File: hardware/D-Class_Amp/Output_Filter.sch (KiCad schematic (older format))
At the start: 4 parts

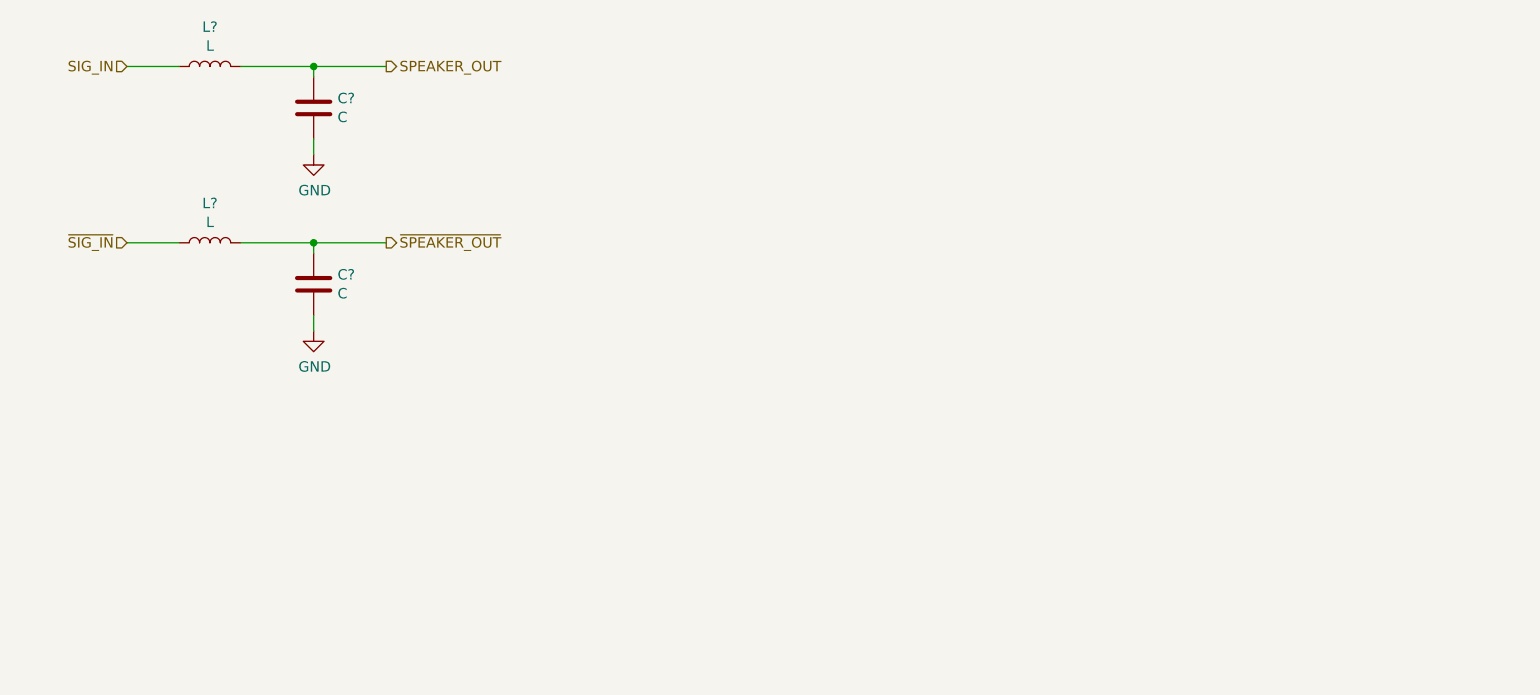
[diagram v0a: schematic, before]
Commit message: single side
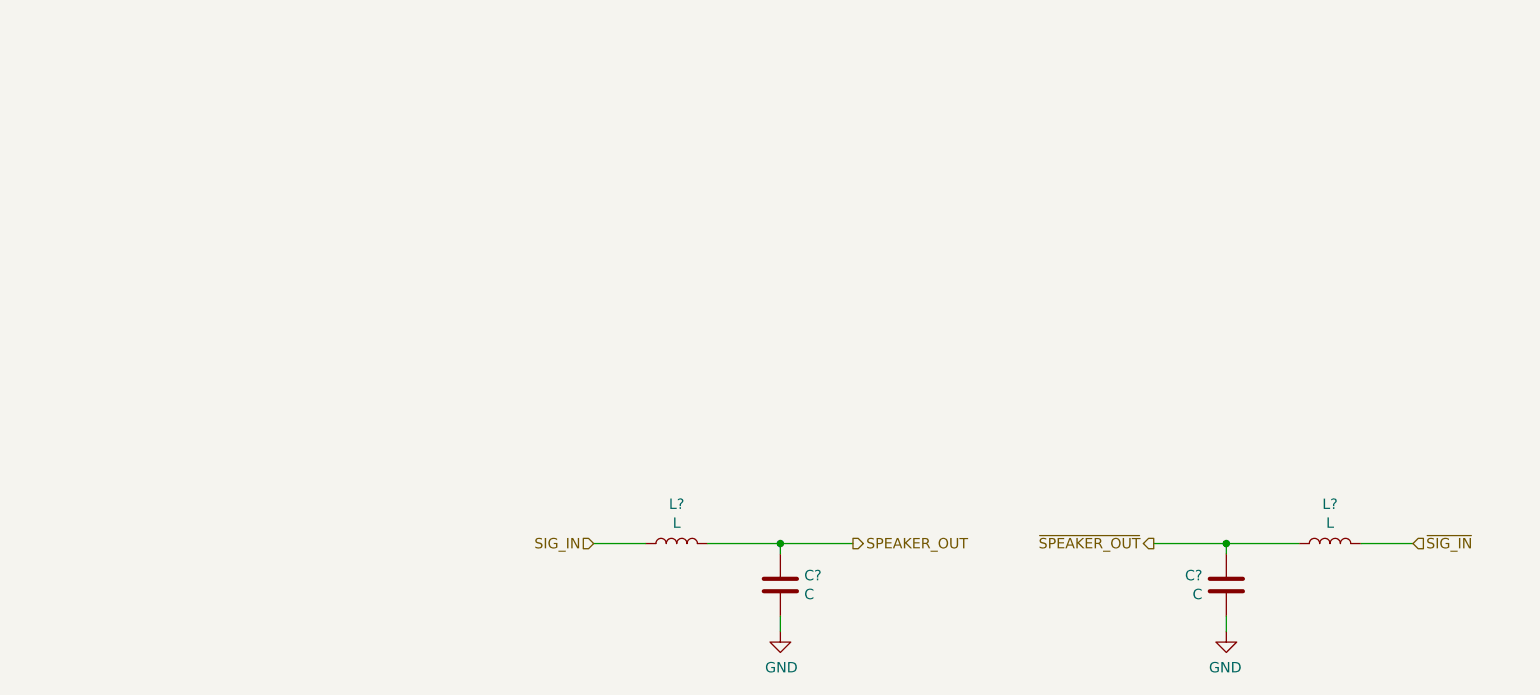
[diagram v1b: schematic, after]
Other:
- moved on the sheet: C?, L?
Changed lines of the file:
@@
 Comment4 ""
 $EndDescr
-Text HLabel 1450 1200 0    50   Input ~ 0
+Text HLabel 3700 3500 0    50   Input ~ 0
 SIG_IN
-Text HLabel 1450 2050 0    50   Input ~ 0
+Text HLabel 7650 3500 2    50   Input ~ 0
 ~SIG_IN
 $Comp
 L Device:L L?
 U 1 1 61193FAD
-P 1850 1200
-F 0 "L?" V 2040 1200 50  0000 C CNN
-F 1 "L" V 1949 1200 50  0000 C CNN
-F 2 "" H 1850 1200 50  0001 C CNN
-F 3 "~" H 1850 1200 50  0001 C CNN
-	1    1850 1200
+P 4100 3500
+F 0 "L?" V 4290 3500 50  0000 C CNN
+F 1 "L" V 4199 3500 50  0000 C CNN
+F 2 "" H 4100 3500 50  0001 C CNN
+F 3 "~" H 4100 3500 50  0001 C CNN
+	1    4100 3500
 	0    -1   -1   0
 $EndComp
@@
 L Device:L L?
 U 1 1 61195264
-P 1850 2050
-F 0 "L?" V 2040 2050 50  0000 C CNN
-F 1 "L" V 1949 2050 50  0000 C CNN
-F 2 "" H 1850 2050 50  0001 C CNN
-F 3 "~" H 1850 2050 50  0001 C CNN
-	1    1850 2050
-	0    -1   -1   0
+P 7250 3500
+F 0 "L?" V 7440 3500 50  0000 C CNN
+F 1 "L" V 7349 3500 50  0000 C CNN
+F 2 "" H 7250 3500 50  0001 C CNN
+F 3 "~" H 7250 3500 50  0001 C CNN
+	1    7250 3500
+	0    1    -1   0
 $EndComp
 $Comp
 L Device:C C?
 U 1 1 611955B4
-P 2350 1400
-F 0 "C?" H 2465 1446 50  0000 L CNN
-F 1 "C" H 2465 1355 50  0000 L CNN
-F 2 "" H 2388 1250 50  0001 C CNN
-F 3 "~" H 2350 1400 50  0001 C CNN
-	1    2350 1400
+P 4600 3700
+F 0 "C?" H 4715 3746 50  0000 L CNN
+F 1 "C" H 4715 3655 50  0000 L CNN
+F 2 "" H 4638 3550 50  0001 C CNN
+F 3 "~" H 4600 3700 50  0001 C CNN
+	1    4600 3700
 	1    0    0    -1
 $EndComp
@@
 L Device:C C?
 U 1 1 61195DF7
-P 2350 2250
-F 0 "C?" H 2465 2296 50  0000 L CNN
-F 1 "C" H 2465 2205 50  0000 L CNN
-F 2 "" H 2388 2100 50  0001 C CNN
-F 3 "~" H 2350 2250 50  0001 C CNN
-	1    2350 2250
-	1    0    0    -1
+P 6750 3700
+F 0 "C?" H 6865 3746 50  0000 L CNN
+F 1 "C" H 6865 3655 50  0000 L CNN
+F 2 "" H 6788 3550 50  0001 C CNN
+F 3 "~" H 6750 3700 50  0001 C CNN
+	1    6750 3700
+	-1   0    0    -1
 $EndComp
 Wire Wire Line
-	1450 1200 1700 1200
+	3700 3500 3950 3500
 Wire Wire Line
-	2000 1200 2350 1200
+	4250 3500 4600 3500
 Wire Wire Line
-	2350 1200 2350 1250
+	4600 3500 4600 3550
 Wire Wire Line
-	2350 1200 2700 1200
-Connection ~ 2350 1200
+	4600 3500 4950 3500
+Connection ~ 4600 3500
 Wire Wire Line
-	1450 2050 1700 2050
+	7650 3500 7400 3500
 Wire Wire Line
-	2000 2050 2350 2050
+	7100 3500 6750 3500
 Wire Wire Line
-	2350 2050 2350 2100
+	6750 3500 6750 3550
 Wire Wire Line
-	2350 2050 2700 2050
-Connection ~ 2350 2050
+	6750 3500 6400 3500
+Connection ~ 6750 3500
 $Comp
 L power:GND #PWR?
 U 1 1 611D879A
-P 2350 1625
-F 0 "#PWR?" H 2350 1375 50  0001 C CNN
-F 1 "GND" H 2355 1452 50  0000 C CNN
-F 2 "" H 2350 1625 50  0001 C CNN
-F 3 "" H 2350 1625 50  0001 C CNN
-	1    2350 1625
+P 4600 3925
+F 0 "#PWR?" H 4600 3675 50  0001 C CNN
+F 1 "GND" H 4605 3752 50  0000 C CNN
+F 2 "" H 4600 3925 50  0001 C CNN
+F 3 "" H 4600 3925 50  0001 C CNN
+	1    4600 3925
 	1    0    0    -1
 $EndComp
@@
 L power:GND #PWR?
 U 1 1 611D8B24
-P 2350 2475
-F 0 "#PWR?" H 2350 2225 50  0001 C CNN
-F 1 "GND" H 2355 2302 50  0000 C CNN
-F 2 "" H 2350 2475 50  0001 C CNN
-F 3 "" H 2350 2475 50  0001 C CNN
-	1    2350 2475
-	1    0    0    -1
+P 6750 3925
+F 0 "#PWR?" H 6750 3675 50  0001 C CNN
+F 1 "GND" H 6755 3752 50  0000 C CNN
+F 2 "" H 6750 3925 50  0001 C CNN
+F 3 "" H 6750 3925 50  0001 C CNN
+	1    6750 3925
+	-1   0    0    -1
 $EndComp
 Wire Wire Line
-	2350 2475 2350 2400
+	6750 3925 6750 3850
 Wire Wire Line
-	2350 1625 2350 1550
-Text HLabel 2700 1200 2    50   Output ~ 0
+	4600 3925 4600 3850
+Text HLabel 4950 3500 2    50   Output ~ 0
 SPEAKER_OUT
-Text HLabel 2700 2050 2    50   Output ~ 0
+Text HLabel 6400 3500 0    50   Output ~ 0
 ~SPEAKER_OUT
 $EndSCHEMATC
